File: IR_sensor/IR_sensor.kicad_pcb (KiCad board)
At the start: 2 copper layers, 13 parts, among them J1 Signal_out, J2 5V_In, J3 GND, J4 5V_In, J5 GND, Q1 BPV11F, U1 LM311P

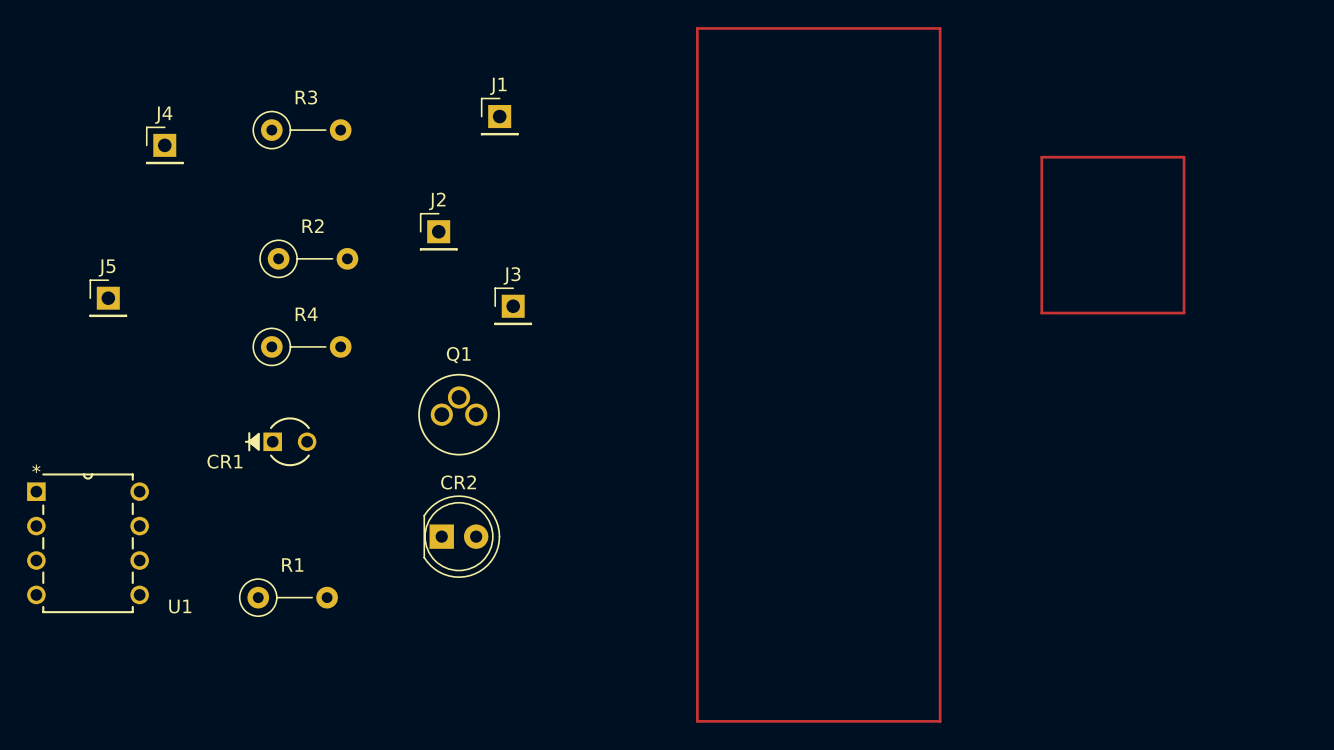
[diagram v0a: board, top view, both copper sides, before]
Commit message: Finalized PCB design
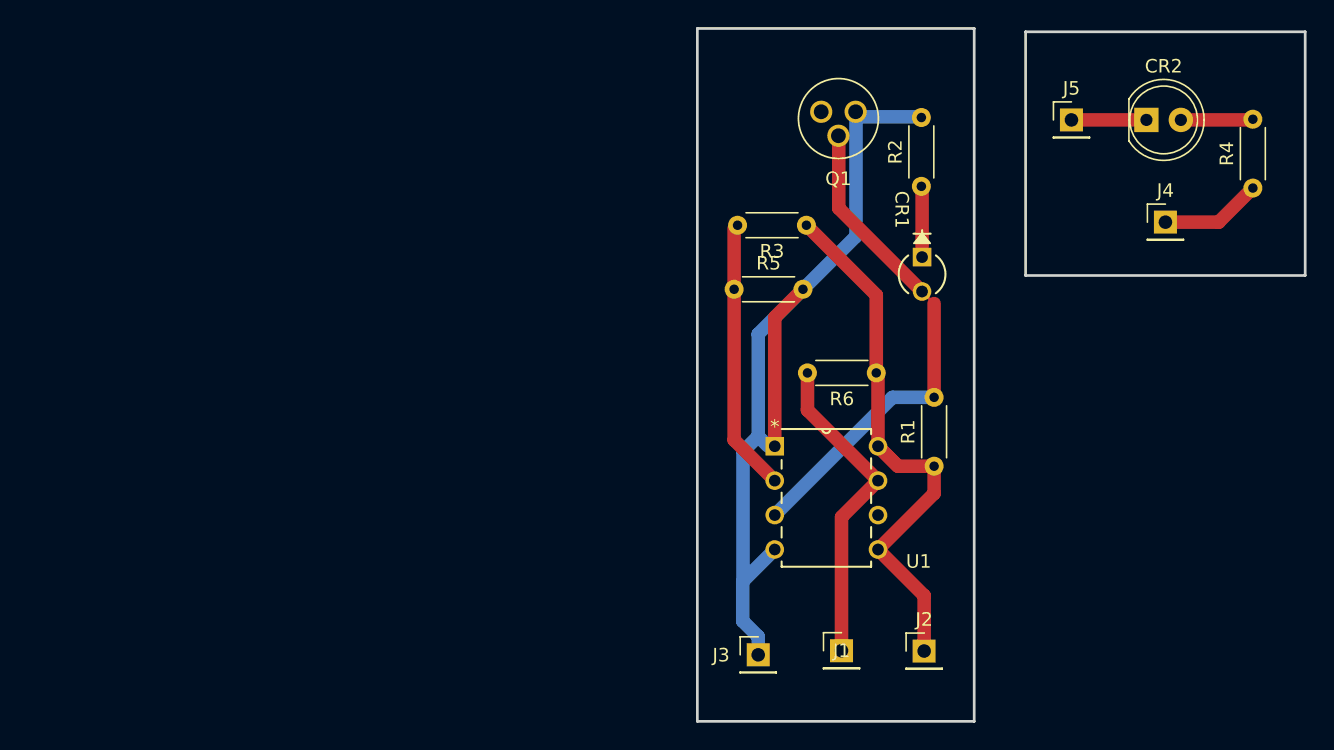
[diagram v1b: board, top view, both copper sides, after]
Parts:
- added R5: 2.2k, Resistor_THT:R_Axial_DIN0204_L3.6mm_D1.6mm_P5.08mm_Horizontal, F.Cu at (133.3, 72.7)
- added R6: 500, Resistor_THT:R_Axial_DIN0204_L3.6mm_D1.6mm_P5.08mm_Horizontal, F.Cu at (143.8, 78.9)
- R1, R2, R4: footprint Resistor_THT:R_Axial_DIN0207_L6.3mm_D2.5mm_P5.08mm_Vertical -> Resistor_THT:R_Axial_DIN0204_L3.6mm_D1.6mm_P5.08mm_Horizontal
- R3: value 1M Ohm -> 3k; footprint Resistor_THT:R_Axial_DIN0207_L6.3mm_D2.5mm_P5.08mm_Vertical -> Resistor_THT:R_Axial_DIN0204_L3.6mm_D1.6mm_P5.08mm_Horizontal
- moved J4 74.1 mm to (165.1, 67.8)
- moved R4 73.3 mm to (171.6, 65.3), turned to 90 degrees
- moved J5 72.3 mm to (158.2, 60.2)
- moved CR2 60.4 mm to (163.7, 60.2)
- moved U1 54.6 mm to (140.4, 88.7)
- moved R1 50.8 mm to (148.1, 85.8), turned to 90 degrees
- moved CR1 49.8 mm to (147.2, 70.4), turned to -90 degrees
- moved R2 47.7 mm to (147.1, 65.2), turned to 90 degrees
- moved J2 47.3 mm to (147.3, 99.4)
- moved J1 46.8 mm to (141.2, 99.4)
- moved R3 40.1 mm to (138.6, 68.0), turned to 180 degrees
- moved Q1 35.5 mm to (141.0, 60.1), turned to 180 degrees
- moved J3 31.4 mm to (135.1, 99.7)
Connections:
- CR1 pad 2: Net-(J1-Pin_1) -> GND
- J2 pad 1: Net-(J2-Pin_1) -> +5V
- J3 pad 1: Net-(J3-Pin_1) -> GND
- Q1 pad C: Net-(J1-Pin_1) -> GND
- Q1 pad E: Net-(J3-Pin_1) -> GND
- R1 pad 1: Net-(J2-Pin_1) -> +5V
- R1 pad 2: Net-(J1-Pin_1) -> GND
- R2 pad 2: Net-(J3-Pin_1) -> GND
- R3 pad 1: Net-(Q1-PadB) -> +5V
- R3 pad 2: GND -> Net-(U1-IN+)
- U1 pad 1: unconnected-(U1-EMITOUT-Pad1) -> GND
- U1 pad 2: unconnected-(U1-IN+-Pad2) -> Net-(U1-IN+)
- U1 pad 3: unconnected-(U1-IN--Pad3) -> GND
- U1 pad 4: unconnected-(U1-VCC--Pad4) -> GND
- U1 pad 5: unconnected-(U1-BALANCE-Pad5) -> +5V
- U1 pad 7: unconnected-(U1-COLOUT-Pad7) -> Net-(J1-Pin_1)
- U1 pad 8: unconnected-(U1-VCC+-Pad8) -> +5V
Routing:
- net GND: track 0.00 -> 103.5 mm
- net +5V: track 0.00 -> 43.9 mm
- net Net-(J1-Pin_1): track 0.00 -> 23.8 mm
- net Net-(U1-IN+): track 0.00 -> 20.2 mm
- net Net-(J4-Pin_1): track 0.00 -> 7.49 mm
- net Net-(J5-Pin_1): track 0.00 -> 5.53 mm
- net Net-(CR2-Pad2): track 0.00 -> 5.33 mm
- net Net-(CR1-Pad1): track 0.00 -> 5.24 mm
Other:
- board outline added: 44.9 x 51.1 mm
